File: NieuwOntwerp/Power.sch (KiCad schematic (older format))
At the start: 44 parts, among them T1 EE13, U10 PC817, U11 TL431, U12 LM1117-3.3, U3 LM358, U5 LM358, U9 LNK364D

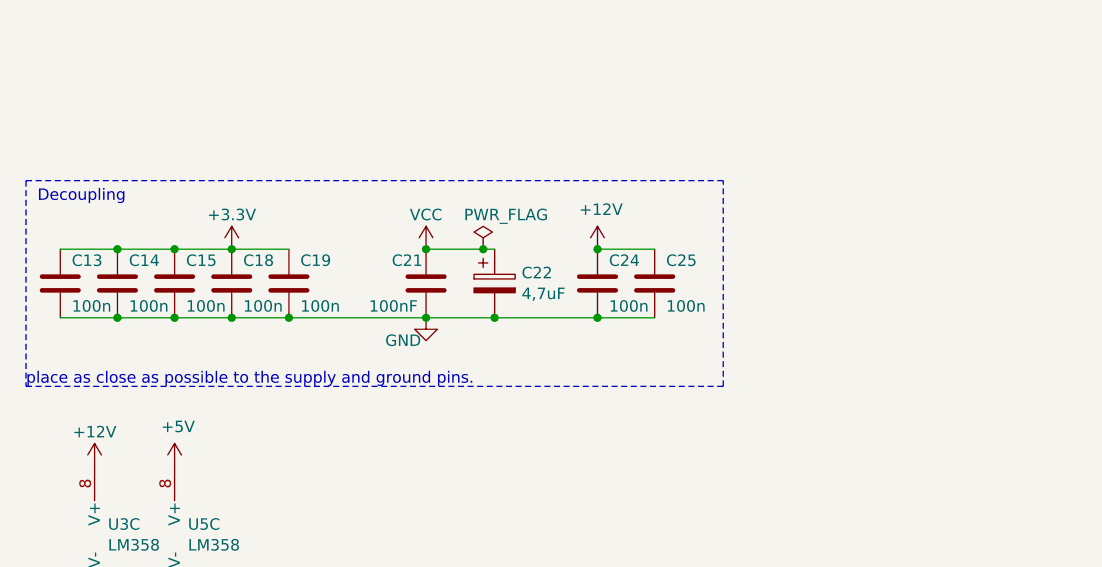
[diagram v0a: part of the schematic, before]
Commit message: 2021-05-15_02
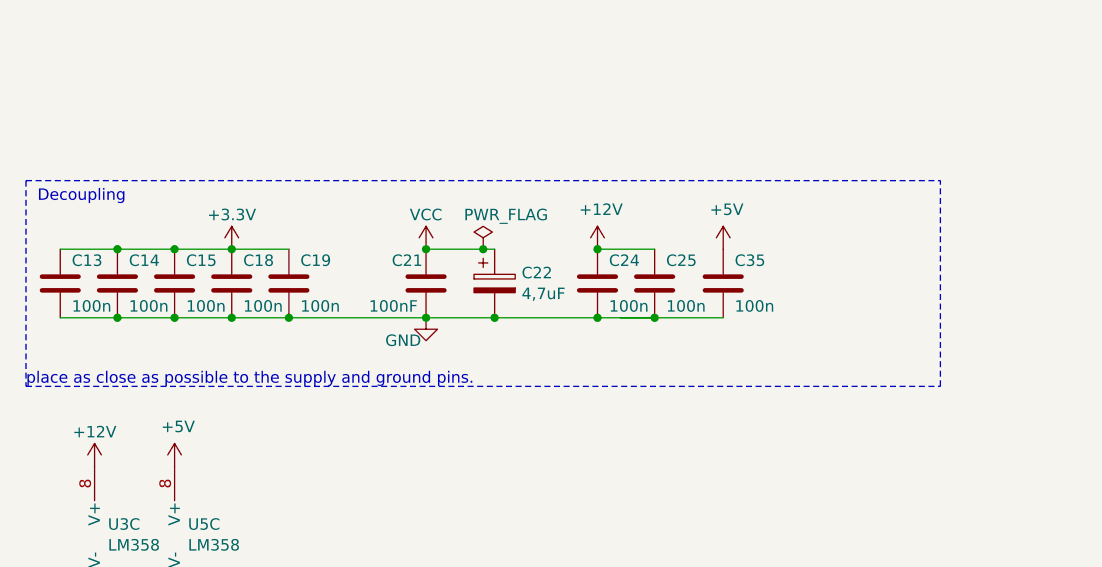
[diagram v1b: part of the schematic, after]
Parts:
- added C35: 100n, Capacitor_SMD:C_0603_1608Metric, symbol Device:C
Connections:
- net +5V: now also C35.2
- net GND: now also C35.1
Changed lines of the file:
@@
 Wire Wire Line
 	3150 4600 3400 4600
-Wire Wire Line
-	3150 4900 3400 4900
 $Comp
 L power:+12V #PWR060
@@
 	650  4300 650  5200
 Wire Notes Line
-	650  5200 3700 5200
-Wire Notes Line
-	3700 5200 3700 4300
-Wire Notes Line
-	3700 4300 650  4300
+	4650 5200 4650 4300
 Text Notes 700  4400 0    50   ~ 0
 Decoupling
@@
 	1    0    0    -1
 $EndComp
+$Comp
+L Device:C C?
+U 1 1 60A477DA
+P 3700 4750
+AR Path="/60A477DA" Ref="C?"  Part="1"
+AR Path="/60357CC4/60A477DA" Ref="C?"  Part="1"
+AR Path="/606C5EA7/60A477DA" Ref="C35"  Part="1"
+F 0 "C35" H 3650 4650 50  0000 R CNN
+F 1 "100n" H 3650 4850 50  0000 R CNN
+F 2 "Capacitor_SMD:C_0603_1608Metric" H 3738 4600 50  0001 C CNN
+F 3 "~" H 3700 4750 50  0001 C CNN
+	1    3700 4750
+	-1   0    0    1
+$EndComp
+Wire Wire Line
+	3700 4900 3400 4900
+Connection ~ 3400 4900
+$Comp
+L power:+5V #PWR042
+U 1 1 60A4B909
+P 3700 4600
+F 0 "#PWR042" H 3700 4450 50  0001 C CNN
+F 1 "+5V" H 3715 4773 50  0000 C CNN
+F 2 "" H 3700 4600 50  0001 C CNN
+F 3 "" H 3700 4600 50  0001 C CNN
+	1    3700 4600
+	1    0    0    -1
+$EndComp
+Wire Wire Line
+	3250 4900 3400 4900
+Wire Notes Line
+	650  4300 4650 4300
+Wire Wire Line
+	3150 4900 3400 4900
+Wire Notes Line
+	650  5200 4650 5200
 $EndSCHEMATC

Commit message: start
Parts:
- removed C14, C18, C25: 100n, Capacitor_SMD:C_0603_1608Metric, symbol Device:C
- added D8: BZT52C-5V1, Diode_SMD:D_SOD-123, symbol Device:D_Zener
- added R57: 1K2, Resistor_SMD:R_0603_1608Metric, symbol Device:R
- added R?: 0R, Resistor_SMD:R_0603_1608Metric, symbol Device:R
- C16, C17: footprint Condensator:JN_102M -> Condensator:Y2_222
- C34: footprint Capacitor_SMD:C_0603_1608Metric -> Condensator:JN_102M
- R48: value 300R -> 330R; footprint Resistor_SMD:R_1210_3225Metric -> Resistor_THT:R_Axial_DIN0207_L6.3mm_D2.5mm_P2.54mm_Vertical
- R49: footprint Resistor_SMD:R_1210_3225Metric -> Resistor_THT:R_Axial_DIN0207_L6.3mm_D2.5mm_P2.54mm_Vertical
- R51: value 150 -> 1K2
- R54: value 6K8 -> 5K6
- T1: footprint Transformers:EE13Horizontal -> Transformers:EE16-A2; symbol Device:Transformer_1P_1S -> Device:Transformer_1P_SS
- U11: value TL431 -> TL432
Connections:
- net +12V: now also R57.1
- net +5V: now also D8.1 (K), R57.2
- net GND: now also T1.2 (AB), D8.2 (A); no longer T1.3 (SA)
- net NEUTRAL: now also D12.4 (~~); no longer D12.1 (+)
- net at C20.1, R47.1: now also D12.3 (~~); no longer D12.2 (-)
- net at C26.1, C27.1, R49.1: now also L1.1, T1.5 (SB); no longer L1.4, T1.1 (AA)
- net at C26.2, C28.2, U9.5 (S)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: now also L1.2; no longer L1.3
- net at D13.2 (A), U9.4 (D): now also T1.3 (SA); no longer T1.2 (AB)
- net at C31.2, R53.2, U11.2 (REF): now also R?.1; no longer R54.1
- net at D14.2 (A), R50.2: now also T1.1 (AA); no longer T1.4 (SB)
- new net: C23.1, D12.1 (+), L1.4
- new net: C23.2, D12.2 (-), L1.3
- new net: R54.1, R?.2
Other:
- note added: "*"
- note added: "* Let op: ondersteboven monteren"
- note added: "Moet meer vermogen zijn"

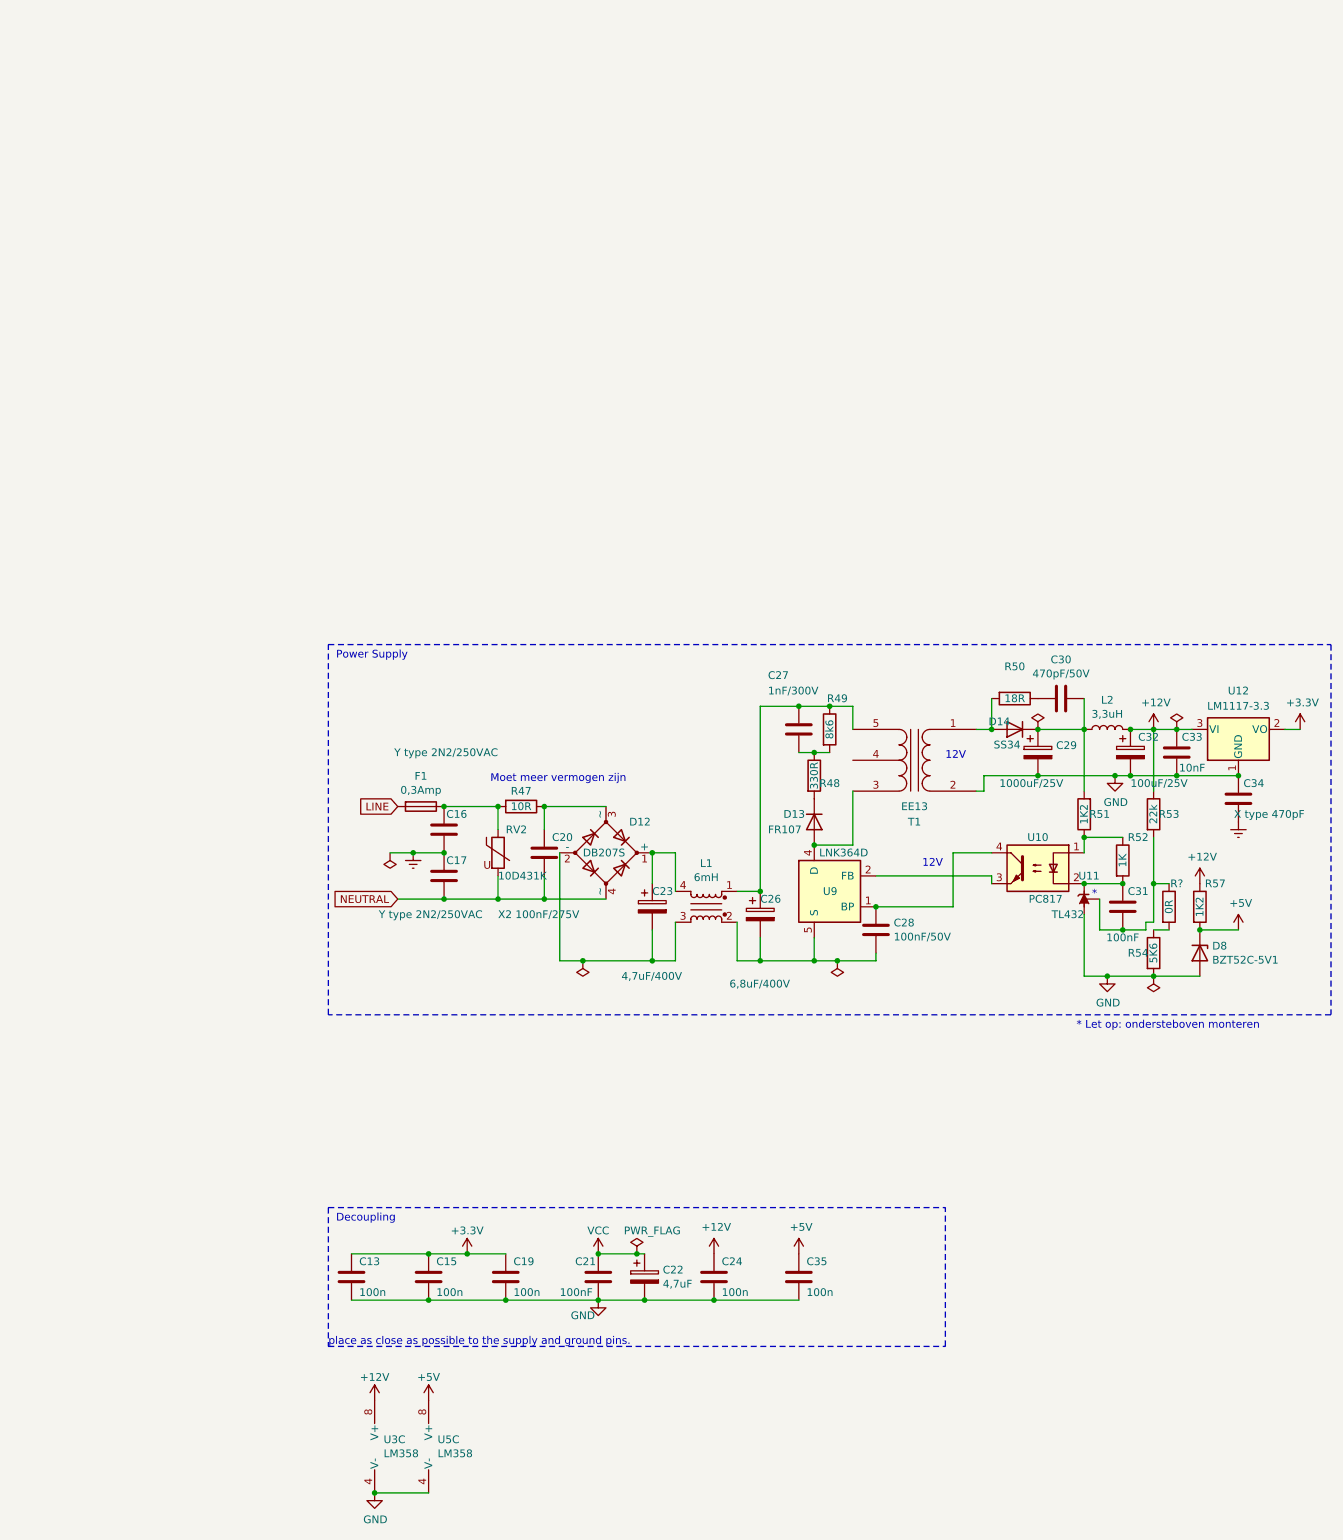
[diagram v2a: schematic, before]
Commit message: Print_update
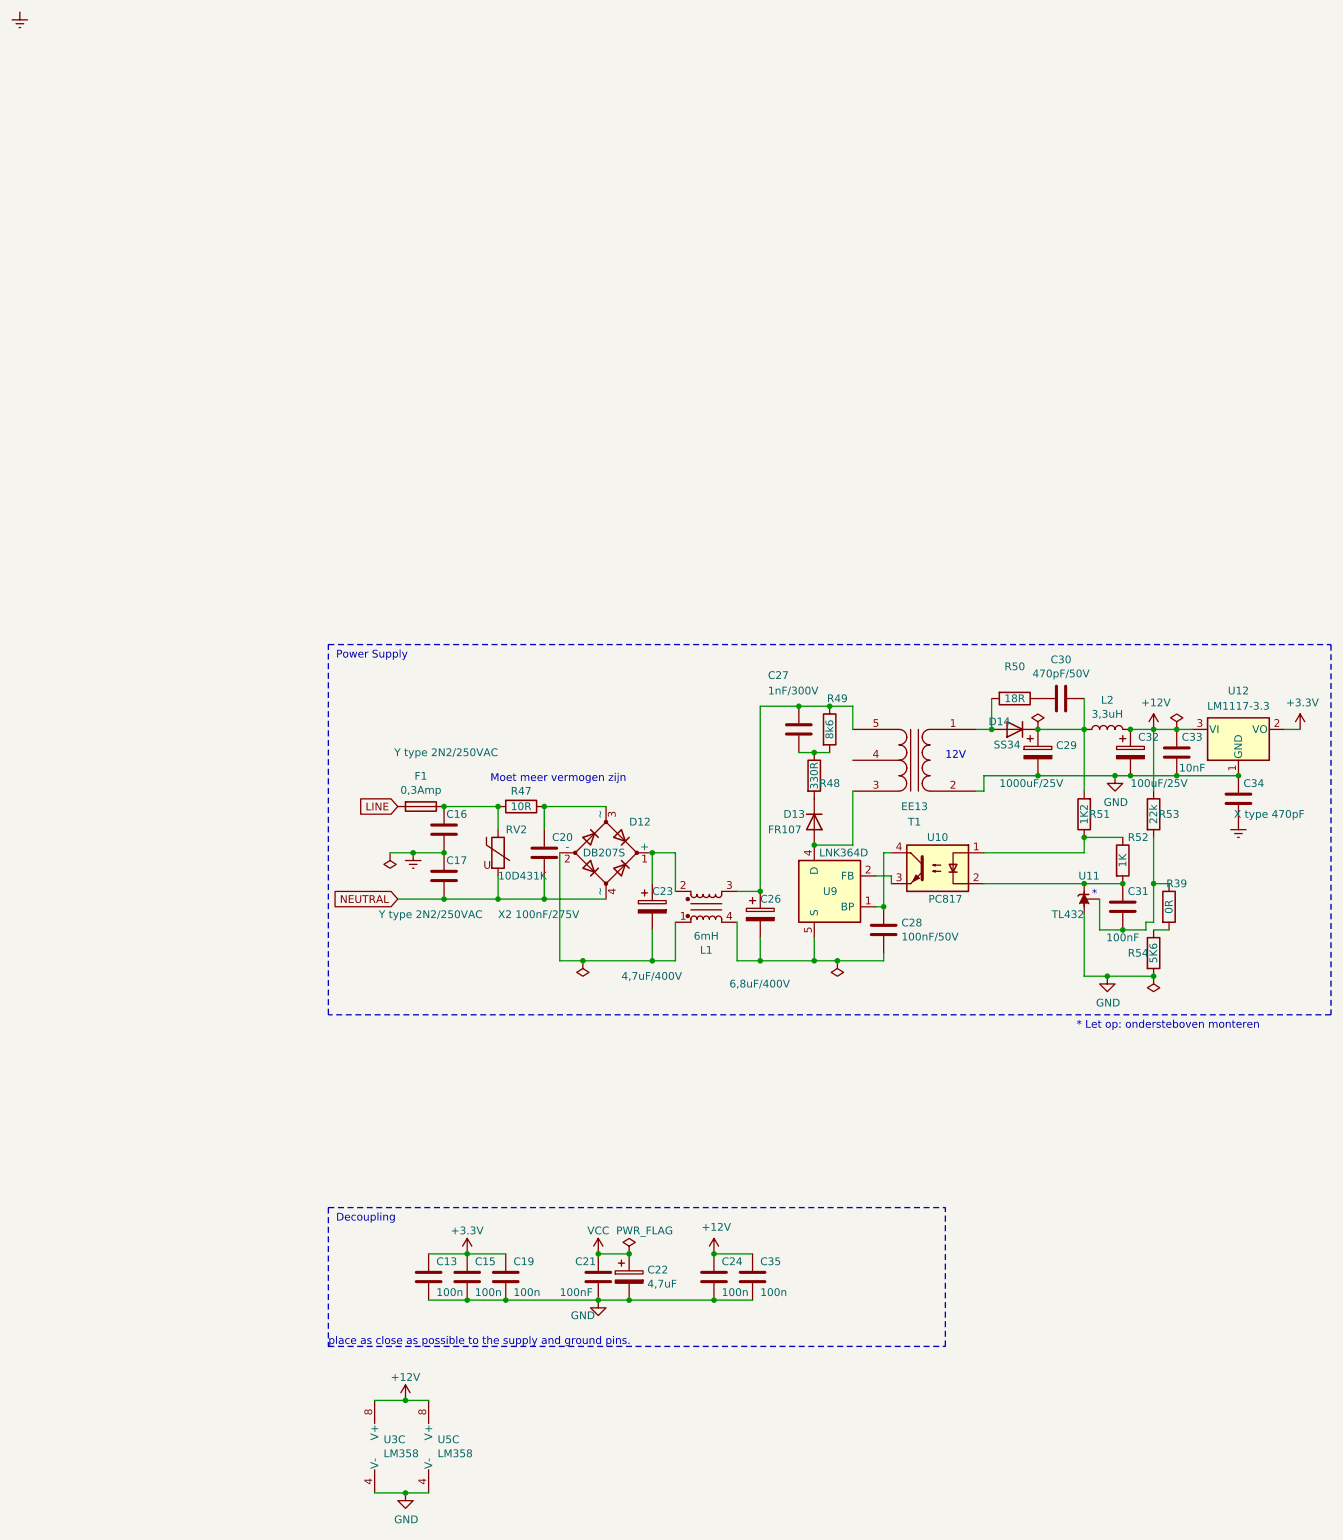
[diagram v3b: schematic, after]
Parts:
- removed D8: BZT52C-5V1, Diode_SMD:D_SOD-123, symbol Device:D_Zener
- removed R57: 1K2, Resistor_SMD:R_0603_1608Metric, symbol Device:R
- F1: footprint Fuse:Fuse_1206_3216Metric -> FuseClip:fuse-clip-5x20mm
- R47: footprint Resistor_SMD:R_2512_6332Metric -> Resistor_THT:R_Axial_DIN0411_L9.9mm_D3.6mm_P5.08mm_Vertical
- gave numbers to parts that had none: 1
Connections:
- net +5V is gone; now on net +12V: C35.2, U5.8 (V+)
- net at C23.1, D12.1 (+): now also L1.2; no longer L1.4
- net at C23.2, D12.2 (-): now also L1.1; no longer L1.3
- net at C26.1, C27.1, R49.1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: now also L1.3; no longer L1.1
- net at C26.2, C28.2, U9.5 (S)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: now also L1.4; no longer L1.2
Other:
- moved on the sheet: C13, C15, C22, C28, C35, U10
